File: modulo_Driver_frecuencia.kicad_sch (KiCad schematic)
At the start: 19 parts, among them J2 Conn_01x02_Pin, Q1 MJE13009G, Q2 MJE13009G, T2 Transformer_1P_1S

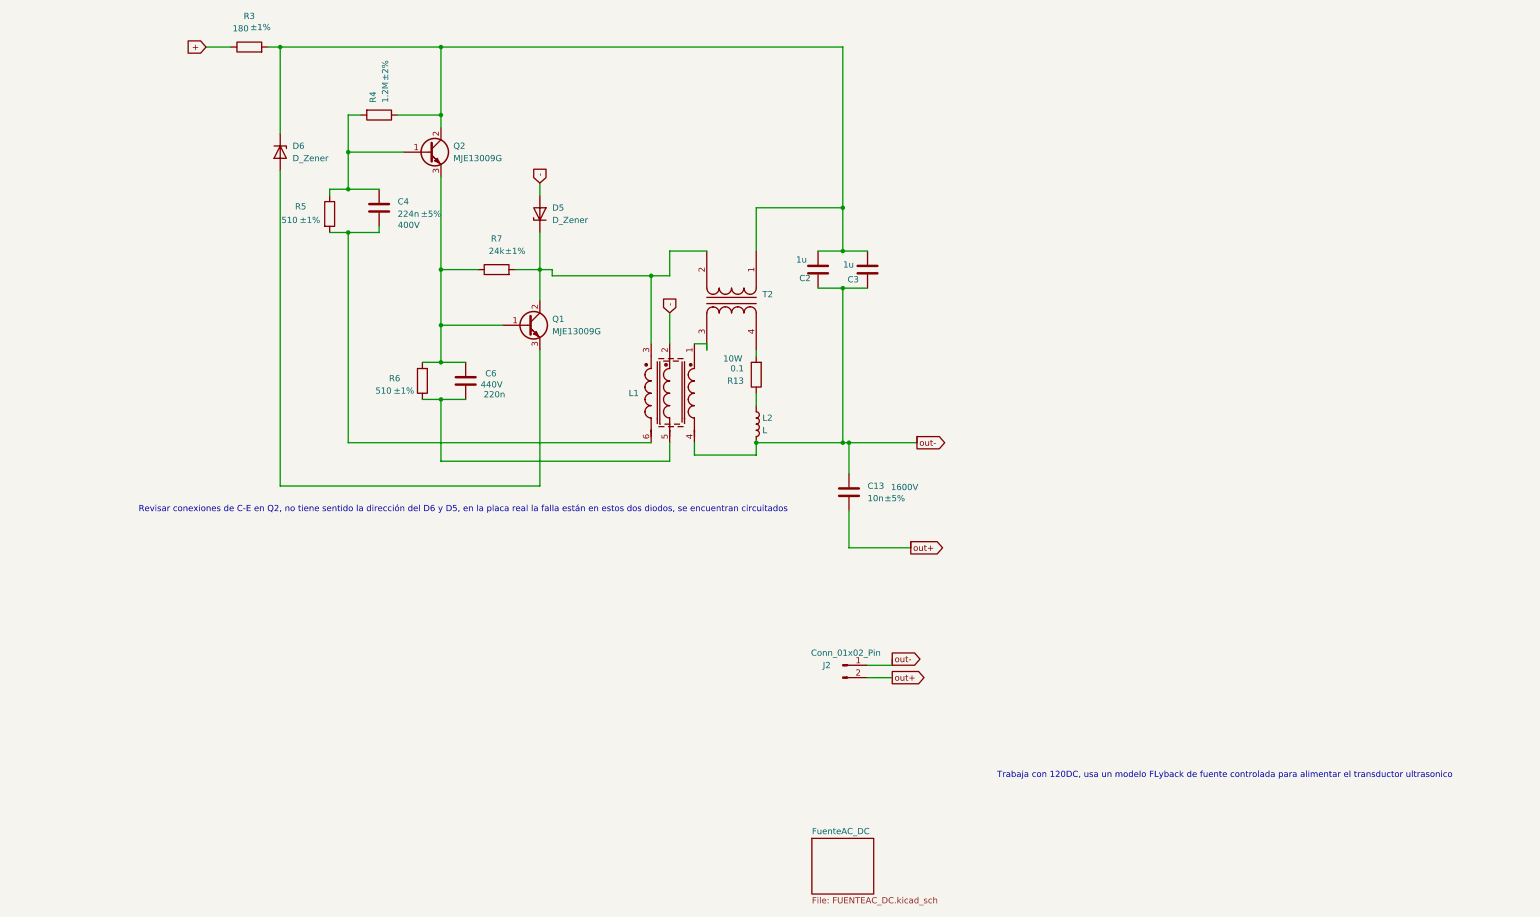
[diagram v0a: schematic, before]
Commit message: 123
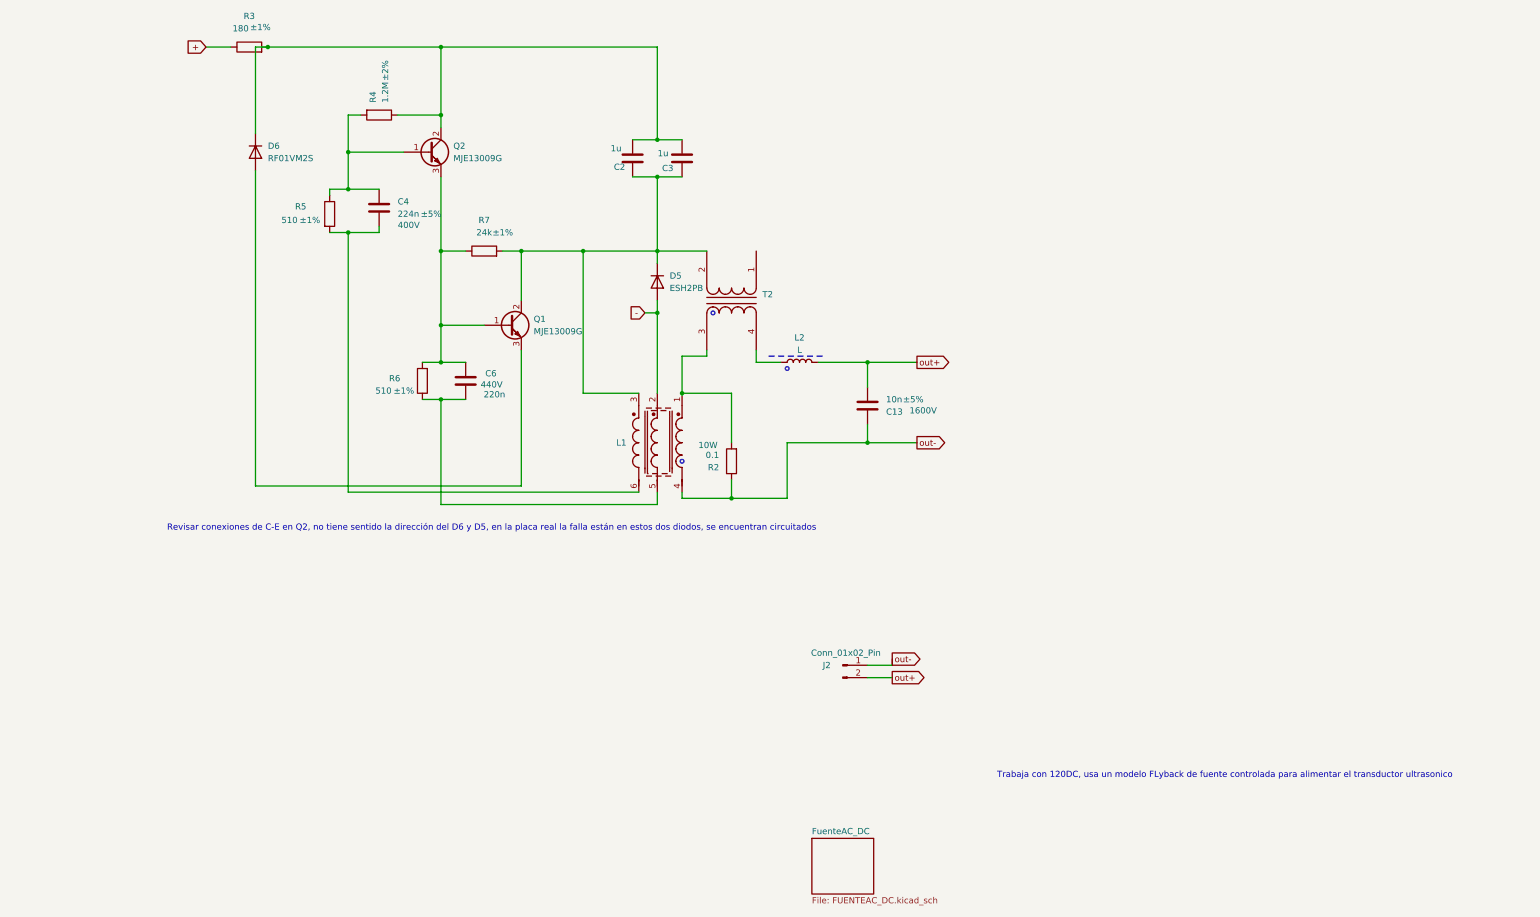
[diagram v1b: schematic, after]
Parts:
- removed D5, D6: D_Zener, symbol Device:D_Zener
- added D5: ESH2PB, Diode_SMD:D_SMP_DO-220AA, symbol Diode:ESH2PB
- added D6: RF01VM2S, Diode_SMD:D_SOD-323, symbol Diode:RF01VM2S
- renumbered R13 to R2
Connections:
- net -: now also D5.2 (A)
- net out+: now also L2.2
- net out-: now also R2.1; no longer C2.1, C3.1, L2.2
- net at C2.2, C3.2, Q2.2 (C)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: now also D6.1 (K); no longer T2.1 (AA)
- net at L1.3, Q1.2 (C), R7.2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: now also C2.1, C3.1, D5.1 (K)
- net at L1.1, T2.3 (SA): now also R2.2
- net at T2.4 (SB): now also L2.1; no longer R2.2
- net at Q1.3 (E): now also D6.2 (A)
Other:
- moved on the sheet: C13, C2, C3, L1, Q1, R2, R7
